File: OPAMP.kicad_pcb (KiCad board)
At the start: 2 copper layers, 49 parts, among them J1 GH125-S02CCA-00, J2 GH125-S06DCA-00, J3 GH125-S03DCA-00, SW1 DSHP02TSGET, U1 ADG704BRMZ-REEL, U2 AD8421BRZ-RL, U3 OPA2197QDGKRQ1, U4 REF2030AIDDCR

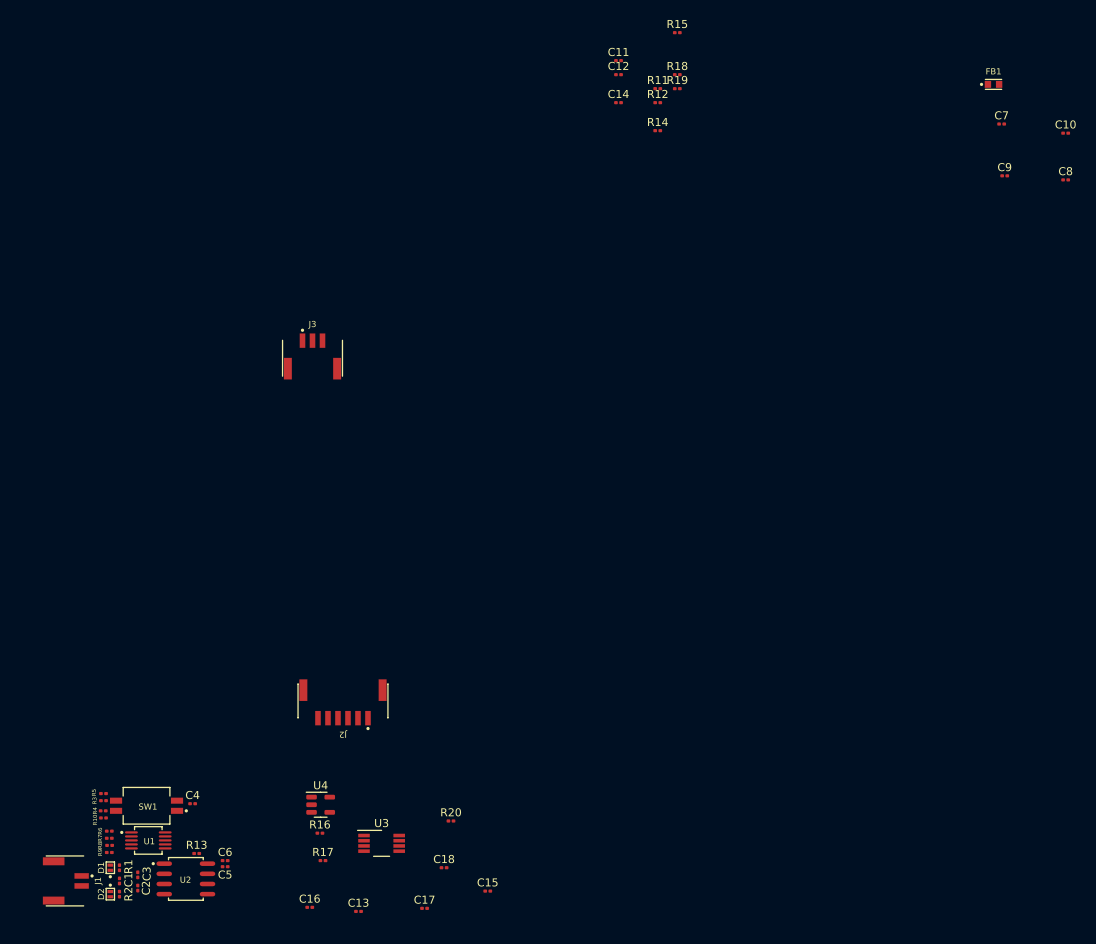
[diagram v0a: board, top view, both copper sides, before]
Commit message: Layout
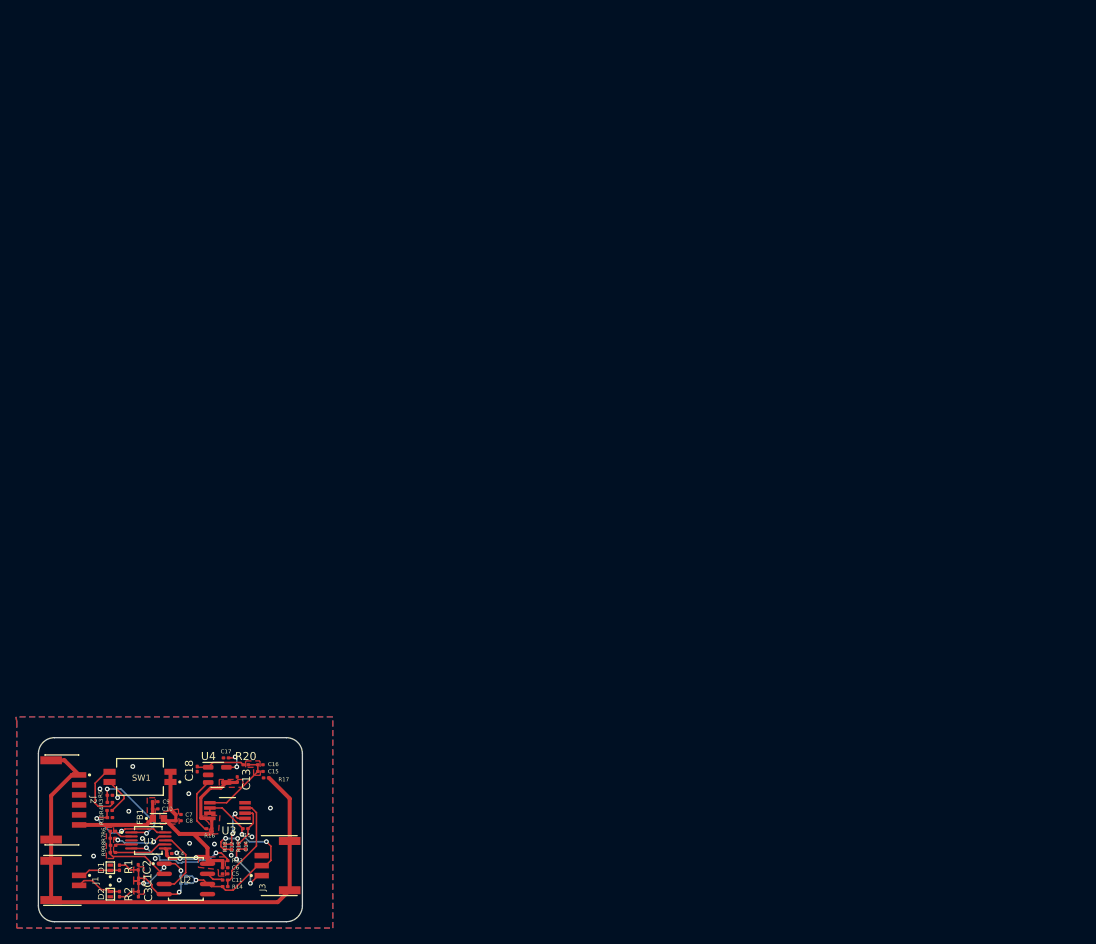
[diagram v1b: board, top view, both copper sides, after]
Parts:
- C11: value 1uF -> 4.7uF
- C12: value 330pF -> 47nF
- R11, R12: value 1M -> 100K; moved to B.Cu
- R14: value 330K -> 68K
- R15: value 4.99K -> 1K
- R18: value 143K -> 28.7K
- R3, R4: value 100 -> 0
- moved C10 141.7 mm to (60.6, 127.9)
- moved FB1 139.0 mm to (61.0, 129.1)
- moved C8 136.8 mm to (63.5, 129.4)
- moved C7 134.3 mm to (63.5, 128.6)
- moved C9 131.9 mm to (60.6, 127.0)
- moved R11 115.7 mm to (64.1, 137.2)
- moved C11 113.6 mm to (69.3, 136.8)
- moved R12 113.4 mm to (64.1, 136.3)
- moved R15 113.2 mm to (71.9, 130.4)
- moved R18 111.9 mm to (69.3, 132.6), turned to -90 degrees
- moved R19 109.5 mm to (71.0, 132.6), turned to -90 degrees
- moved R14 108.9 mm to (69.3, 137.6), turned to 180 degrees
- moved C12 107.9 mm to (70.2, 132.6), turned to -90 degrees
- moved C14 104.0 mm to (71.9, 132.6), turned to 90 degrees
- moved J3 64.0 mm to (75.7, 135.0), turned to 90 degrees
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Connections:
- net /COIL_N_FILT renamed /COIL_FILT_N
- net /COIL_N_RAW renamed /COIL_RAW_N
- net /COIL_P_FILT renamed /COIL_FILT_P
- net /COIL_P_RAW renamed /COIL_RAW_P
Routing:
- net /AGND_SHIELD: track 0.00 -> 67.5 mm
- net +5VA: track 0.00 -> 39.0 mm, vias 0 -> 2
- net /BIAS_1V5: track 0.00 -> 27.5 mm, vias 0 -> 3
- net Net-(U1-EN): track 0.00 -> 14.2 mm, vias 0 -> 2
- net Net-(U1-A0): track 0.00 -> 13.0 mm, vias 0 -> 2
- net /HP_IN: track 0.00 -> 12.5 mm
- net Net-(U1-A1): track 0.00 -> 12.0 mm, vias 0 -> 2
- net /+5VIN: track 0.00 -> 11.7 mm
- net /COIL_FILT_N: track 0.00 -> 11.4 mm, vias 0 -> 3
- net /COIL_FILT_P: track 0.00 -> 11.0 mm, vias 0 -> 1
- net /VOUT_RAW: track 0.00 -> 10.7 mm, vias 0 -> 2
- net /RG_A: track 0.00 -> 10.7 mm
- net /BIAS_FILT: track 0.00 -> 9.66 mm
- net /RG_B: track 0.00 -> 8.83 mm
- net /VOUT: track 0.00 -> 7.80 mm, vias 0 -> 2
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- added copper zone on F.Cu, net +5VA
- added copper zone on F.Cu, net /+5VIN
- added copper zone on B.Cu, net /AGND
- added copper zone on F.Cu, net /AGND
- added copper zone on F.Cu, net /BIAS_FILT
- added copper zone on F.Cu, net /COIL_FILT_N
- added copper zone on F.Cu, net /COIL_FILT_P
- added copper zone on F.Cu, net /RG_A
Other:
- board outline added: 33 x 23 mm
